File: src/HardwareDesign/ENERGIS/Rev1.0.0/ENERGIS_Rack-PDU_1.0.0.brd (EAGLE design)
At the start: 210 x 108 mm, 402 parts, among them IC1 MP2315GJ-Z, IC10 HLW8032, IC11 HLW8032, IC12 HLW8032, IC13 MP150GJ, IC14 HLW8032, IC15 RP2040, IC16 HLW8032, IC17 MCP6001RT-I/OT, IC18 W25Q128JVPIQ, IC19 CAT24C256HU4IGT3, IC2 MP2315GJ-Z, IC20 W5500, IC21 MIC5504-3.3YM5, IC22 MCP6001RT-I/OT, IC3 ULN2803AFWG, IC4 MCP23017T-E/ML, IC5 MP150GJ, IC6 HLW8032, IC7 HLW8032, IC8 HLW8032, IC9 SN74HC151PWR, J10 0R 1%, J2 JP, J7 JP, J8 0R 1%, J9 0R 1%, K1 G2RL-1A-E DC12, K2 G2RL-1A-E DC12, K3 G2RL-1A-E DC12, K4 G2RL-1A-E DC12, K5 G2RL-1A-E DC12, K6 G2RL-1A-E DC12, K7 G2RL-1A-E DC12, K8 G2RL-1A-E DC12, P12ON Green, P3ON Green, P5ON Green, SW3 TP, X1 12MHz, X2 25MHz

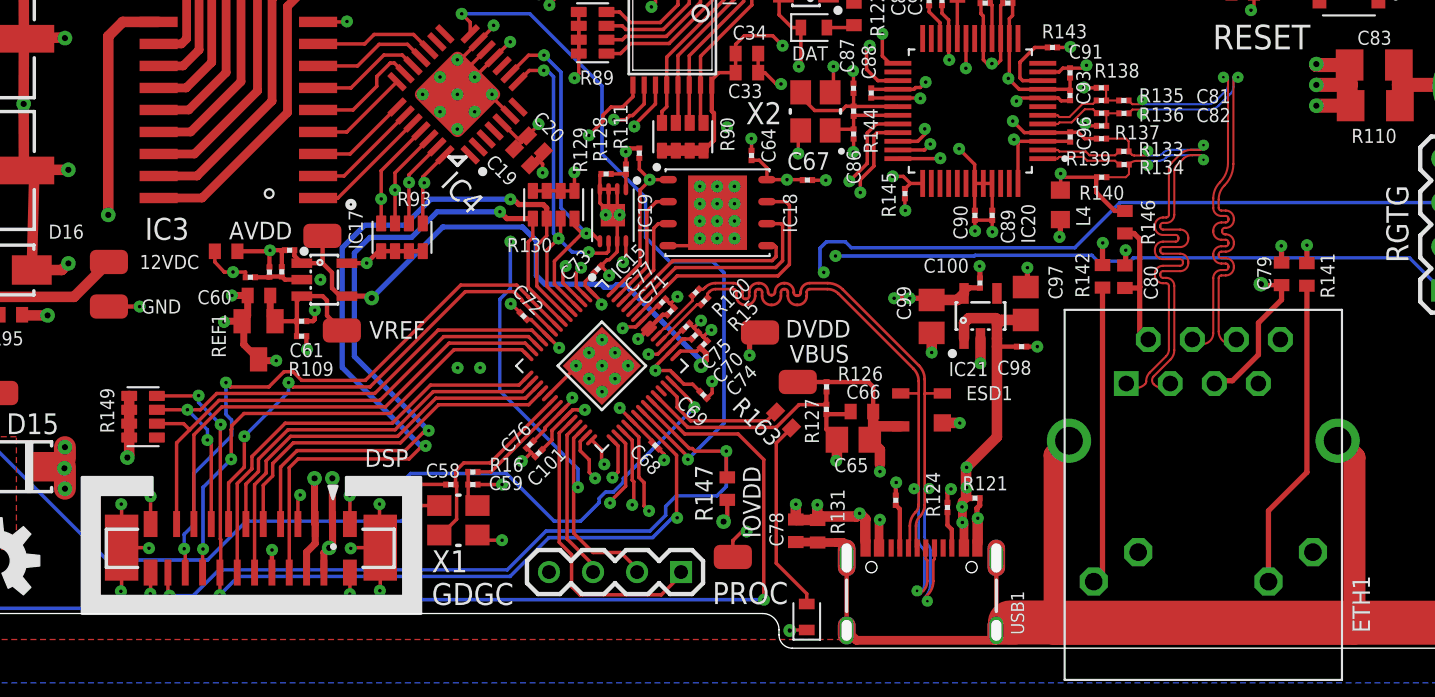
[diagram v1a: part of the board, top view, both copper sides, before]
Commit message: update software, bugfix
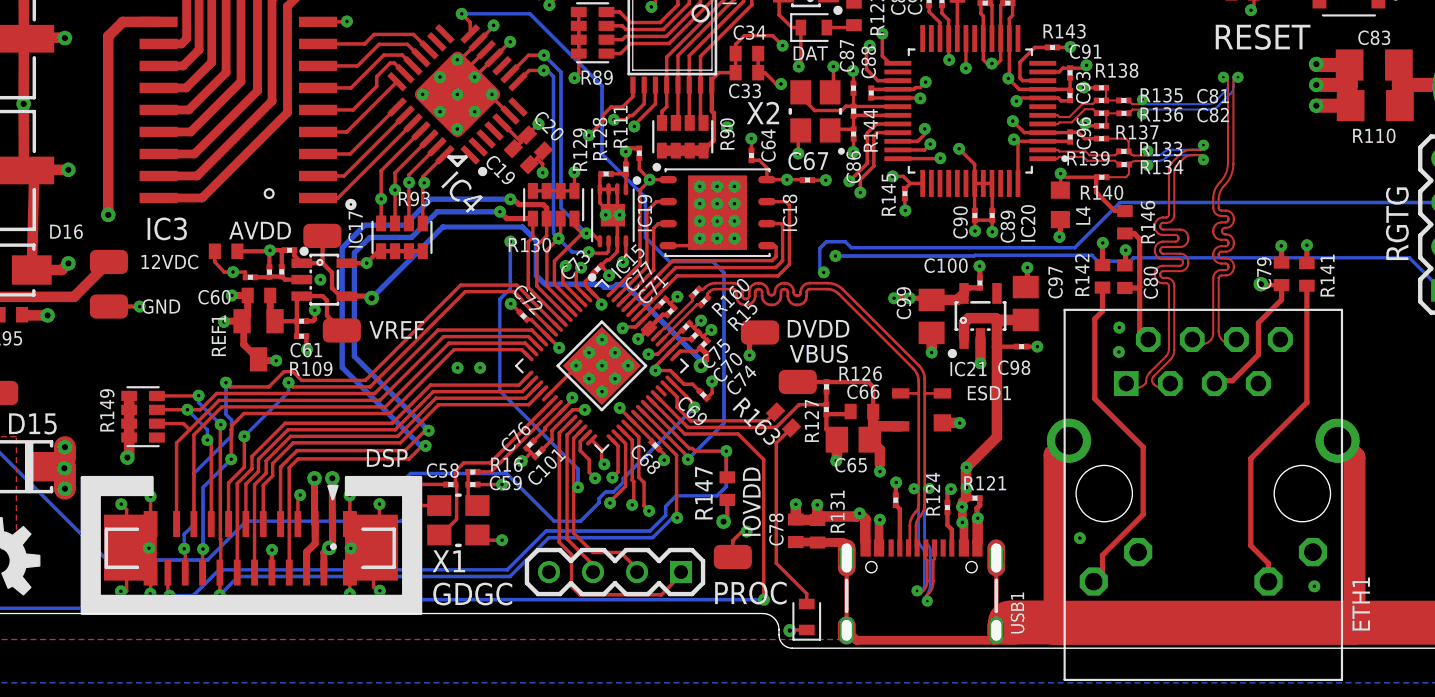
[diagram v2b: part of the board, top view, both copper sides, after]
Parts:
- R93: value 4x10K 1206 -> 10K 1%; device Resistor Array:742C083103JP -> ds_resistor:_0603X4-1206
- X1: value 12MHz -> ABM8-272-T3 12MHz
- moved C19 0.07 mm to (152.1, 26.4)
- moved C20 0.05 mm to (152.9, 27.1)
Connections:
- net GND: now also R93.A2, R93.B2, R93.C2, R93.D2; no longer R93.5, R93.6, R93.7, R93.8
- net MUX_A: now also R93.D1; no longer R93.4
- net MUX_B: now also R93.C1; no longer R93.3
- net MUX_C: now also R93.B1; no longer R93.2
- net MUX_EN: now also R93.A1; no longer R93.1
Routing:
- net N$91: track 17.2 -> 19.5 mm
- net N$82: track 18.0 -> 18.8 mm
- net GND: vias 151 -> 155

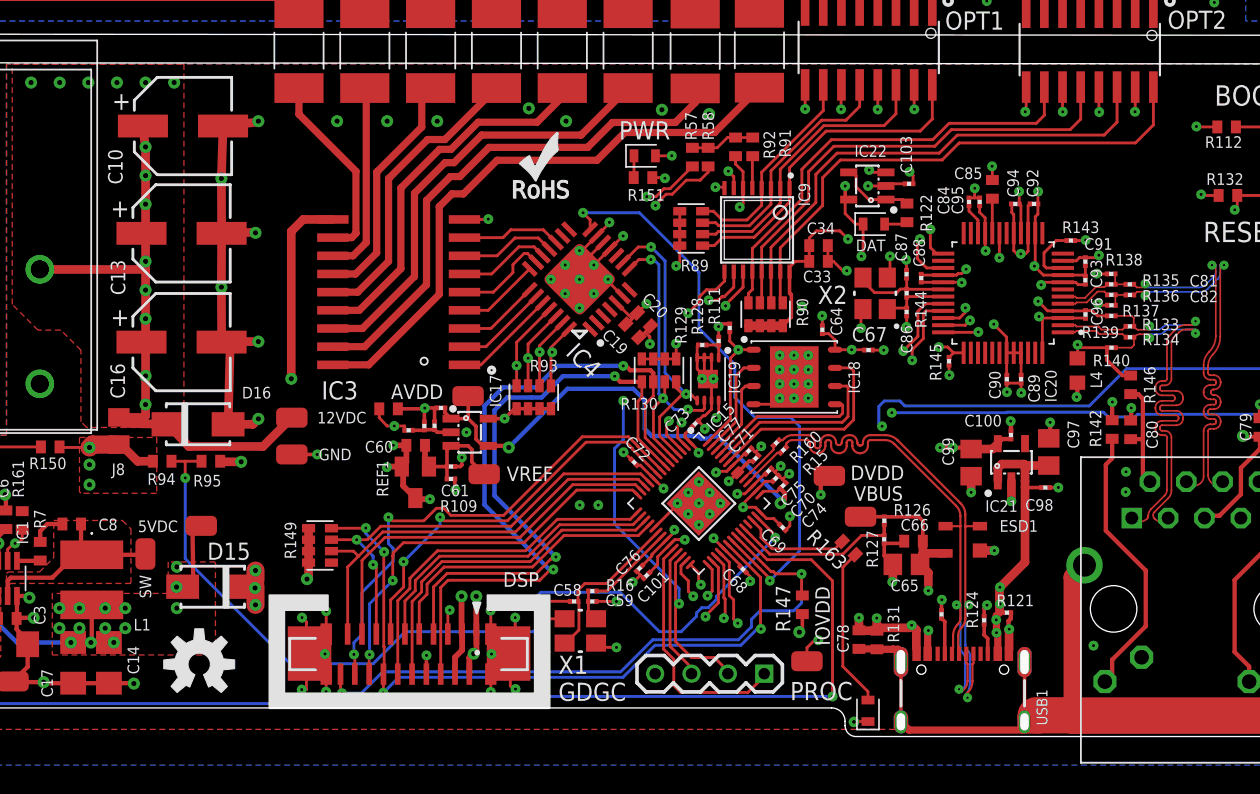
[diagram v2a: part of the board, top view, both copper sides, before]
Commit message: Baseline commit. Device is functioning as expected, software is working
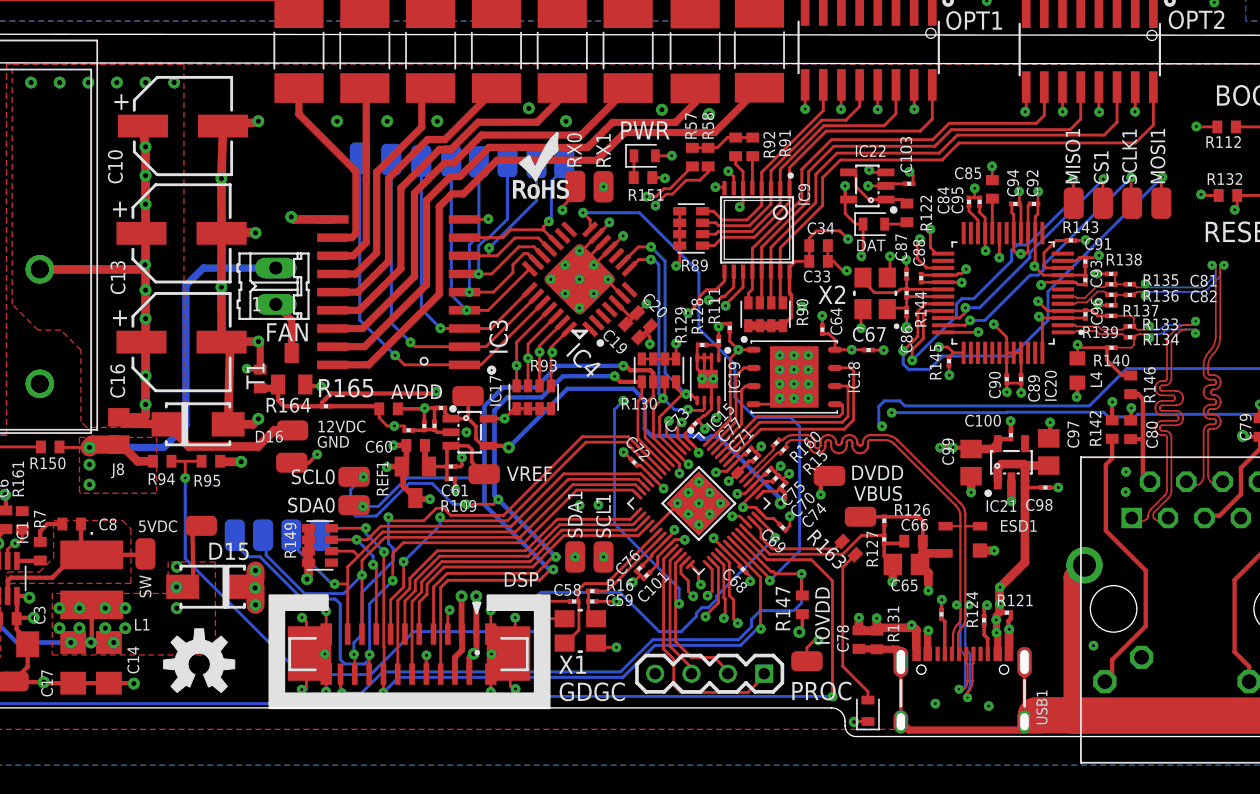
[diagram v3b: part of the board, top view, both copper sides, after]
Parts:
- added CS0, CS1, MISO0, MISO1, MOSI0, MOSI1, REL0, REL1, REL2, REL3, REL4, REL5, REL6, REL7, RX0, RX1, SCL0, SCL1, SCLK0, SCLK1, SDA0, SDA1: TP, ds_passive:TP
- added FAN: (no value), con-amp-quick:02P
- added R164: 10K 1%, ds_resistor:0402
- added R165: NC, ds_passive:R0201
- added T1: (no value), ds_active:SOT23
- moved 12VDC 0.89 mm to (128.4, 19.4)
- moved GND 0.58 mm to (128.3, 17.1)
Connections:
- new net FAN_CTRL: IC15.39, R164.1, R165.1, T1.1
- new net N$23: FAN.1, T1.3
- net !W5500_CS: now also CS1.TP
- net +12V: now also FAN.2
- net +3V3_MCU: now also R165.2
- net GND: now also R164.2, T1.2
- net I2C0_SCL: now also SCL0.TP
- net I2C0_SDA: now also SDA0.TP
- net I2C1_SCL: now also SCL1.TP
- net I2C1_SDA: now also SDA1.TP
- net LCD_CS: now also CS0.TP
- net LCD_MISO: now also MISO0.TP
- net LCD_MOSI: now also MOSI0.TP
- net LCD_SCLK: now also SCLK0.TP
- net REL_0: now also REL0.TP
- net REL_1: now also REL1.TP
- net REL_2: now also REL2.TP
- net REL_3: now also REL3.TP
- net REL_4: now also REL4.TP
- net REL_5: now also REL5.TP
- net REL_6: now also REL6.TP
- net REL_7: now also REL7.TP
- net UART0_RX: now also RX0.TP
- net UART0_TX: now also RX1.TP
- net W5500_MISO: now also MISO1.TP
- net W5500_MOSI: now also MOSI1.TP
- net W5500_SCK: now also SCLK1.TP
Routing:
- net FAN_CTRL: track 0.00 -> 50.1 mm, vias 0 -> 2
- net !W5500_CS: track 33.8 -> 61.5 mm, vias 2 -> 3
- net +12V: track 370.5 -> 395.1 mm
- net REL_7: track 7.27 -> 27.2 mm, vias 0 -> 1
- net W5500_SCK: track 33.9 -> 53.8 mm, vias 2 -> 3
- net W5500_MOSI: track 40.0 -> 57.4 mm, vias 2 -> 3
- net REL_6: track 6.47 -> 23.7 mm, vias 0 -> 1
- net LCD_MOSI: track 28.2 -> 44.4 mm
- net I2C0_SCL: track 43.0 -> 58.6 mm, vias 2 -> 5
- net W5500_MISO: track 39.7 -> 55.0 mm, vias 2 -> 3
- net REL_5: track 5.68 -> 19.6 mm, vias 0 -> 1
- net I2C1_SDA: track 21.4 -> 35.1 mm, vias 2 -> 4
- net REL_4: track 5.76 -> 16.6 mm, vias 0 -> 1
- net I2C1_SCL: track 22.1 -> 32.6 mm, vias 3 -> 5
- net I2C0_SDA: track 48.4 -> 58.4 mm, vias 2 -> 3
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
